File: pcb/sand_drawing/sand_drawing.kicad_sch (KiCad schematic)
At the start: 39 parts, among them J0 12V GND, J1 Stepper1, J2 Stepper2, J3 Opto 1, J4 Opto 2, J5 UART, SW1 EN, SW2 IO0, U2 AMS1117-3.3, U3 ESP32-WROOM-32D

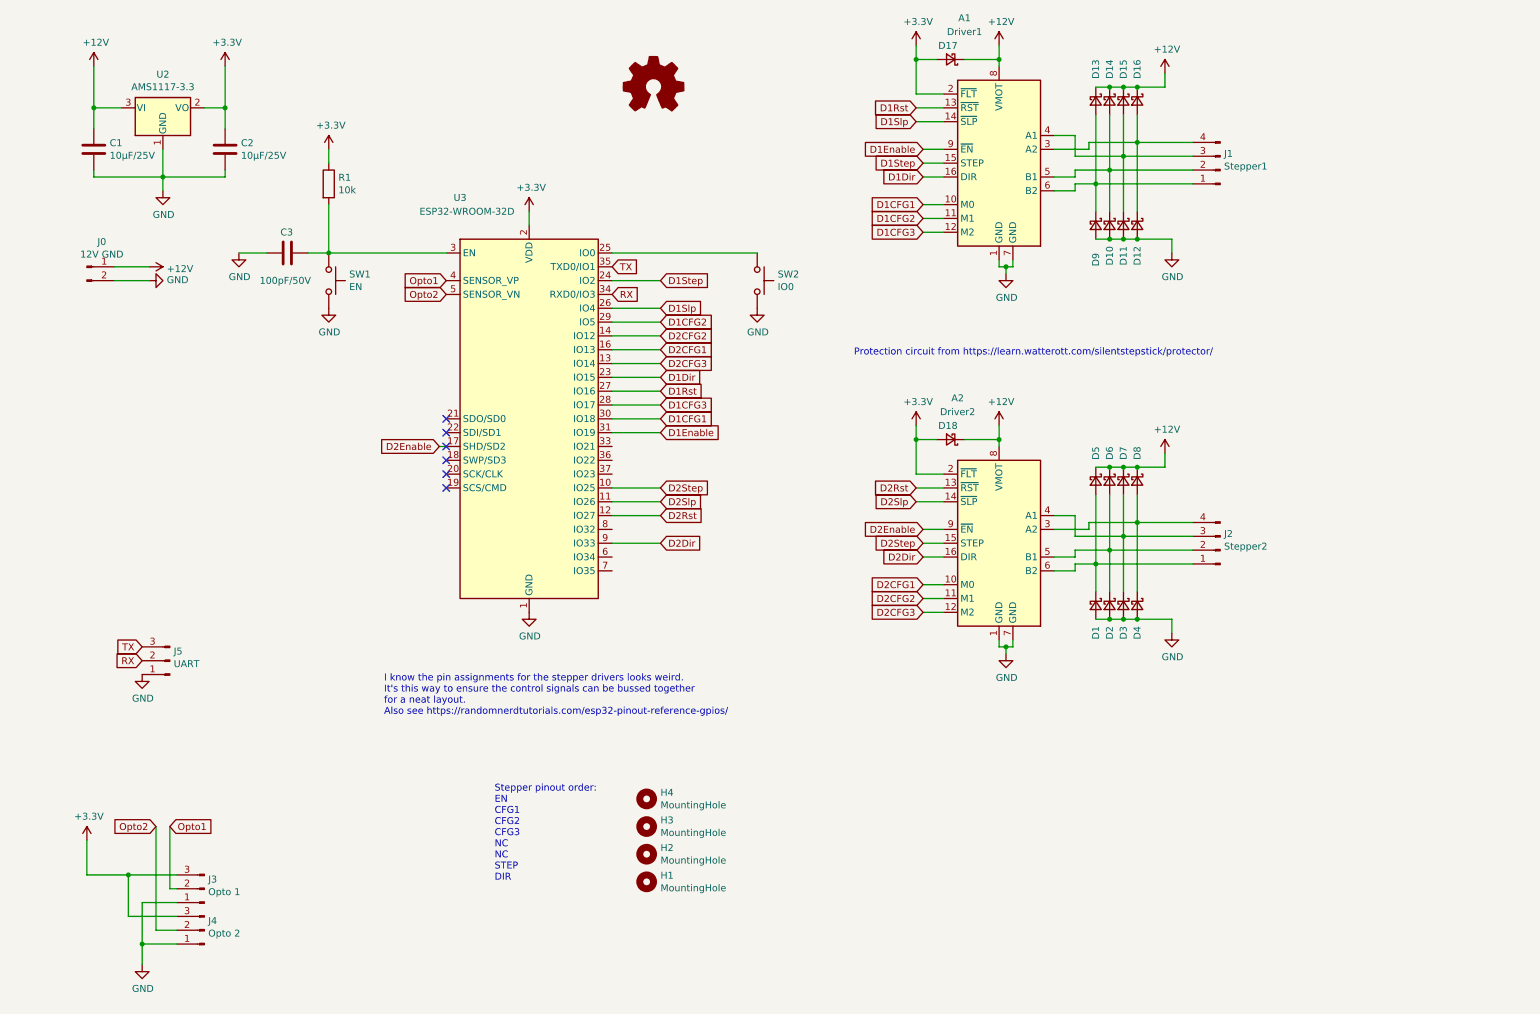
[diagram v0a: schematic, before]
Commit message: Working on new vreg
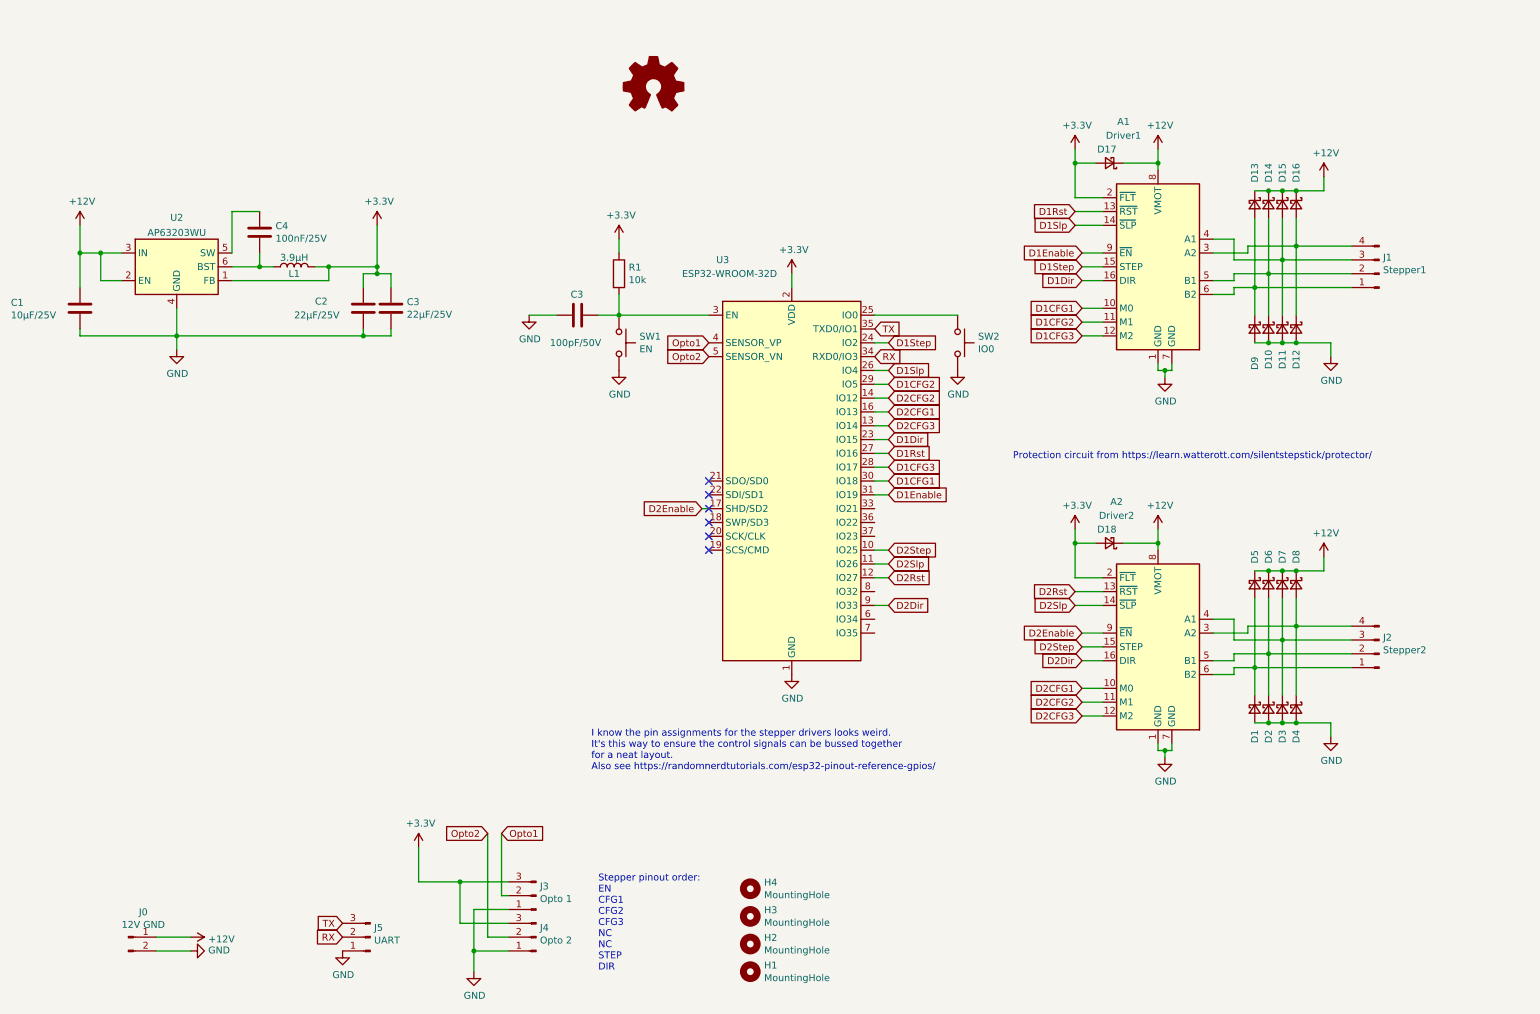
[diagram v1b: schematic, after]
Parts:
- removed U2: AMS1117-3.3, Package_TO_SOT_SMD:SOT-223, symbol Regulator_Linear:LD1117S33TR_SOT223
- added C3: 22µF/25V, Capacitors_SMD:C_1206, symbol Device:C
- added C4: 100nF/25V, Capacitors_SMD:C_1206, symbol Device:C
- added L1: 3.9µH, symbol Device:L
- added U2: AP63203WU, Package_TO_SOT_SMD:TSOT-23-6, symbol Regulator_Switching:AP63203WU
- C1: footprint Capacitors_SMD:C_0805 -> Capacitors_SMD:C_1206
- C2: value 10µF/25V -> 22µF/25V; footprint Capacitors_SMD:C_0805 -> Capacitors_SMD:C_1206
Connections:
- net +12V: now also U2.2 (EN), U2.3 (IN)
- net +3V3: now also C3.1, L1.2, U2.1 (FB)
- net GND: now also C3.2, U2.4 (GND)
- new net: C4.1, U2.5 (SW)
- new net: C4.2, L1.1, U2.6 (BST)
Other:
- moved on the sheet: A1, A2, C1, C2, C3, D1, D10, D11, D12, D13, D14, D15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
